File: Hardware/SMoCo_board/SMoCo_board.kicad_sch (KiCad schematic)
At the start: 37 parts, among them J1 Conn_01x02, J2 Conn_01x02, J3 Conn_01x02, J4 Conn_01x02, J5 Conn_01x06, J6 Conn_01x02, J7 Conn_01x04, J8 Conn_01x02, Q1 Q_PMOS, U1 STM32F072C8T6, U2 VNH7040AYTR, U3 SN65HVD232, U4 AP63203WU

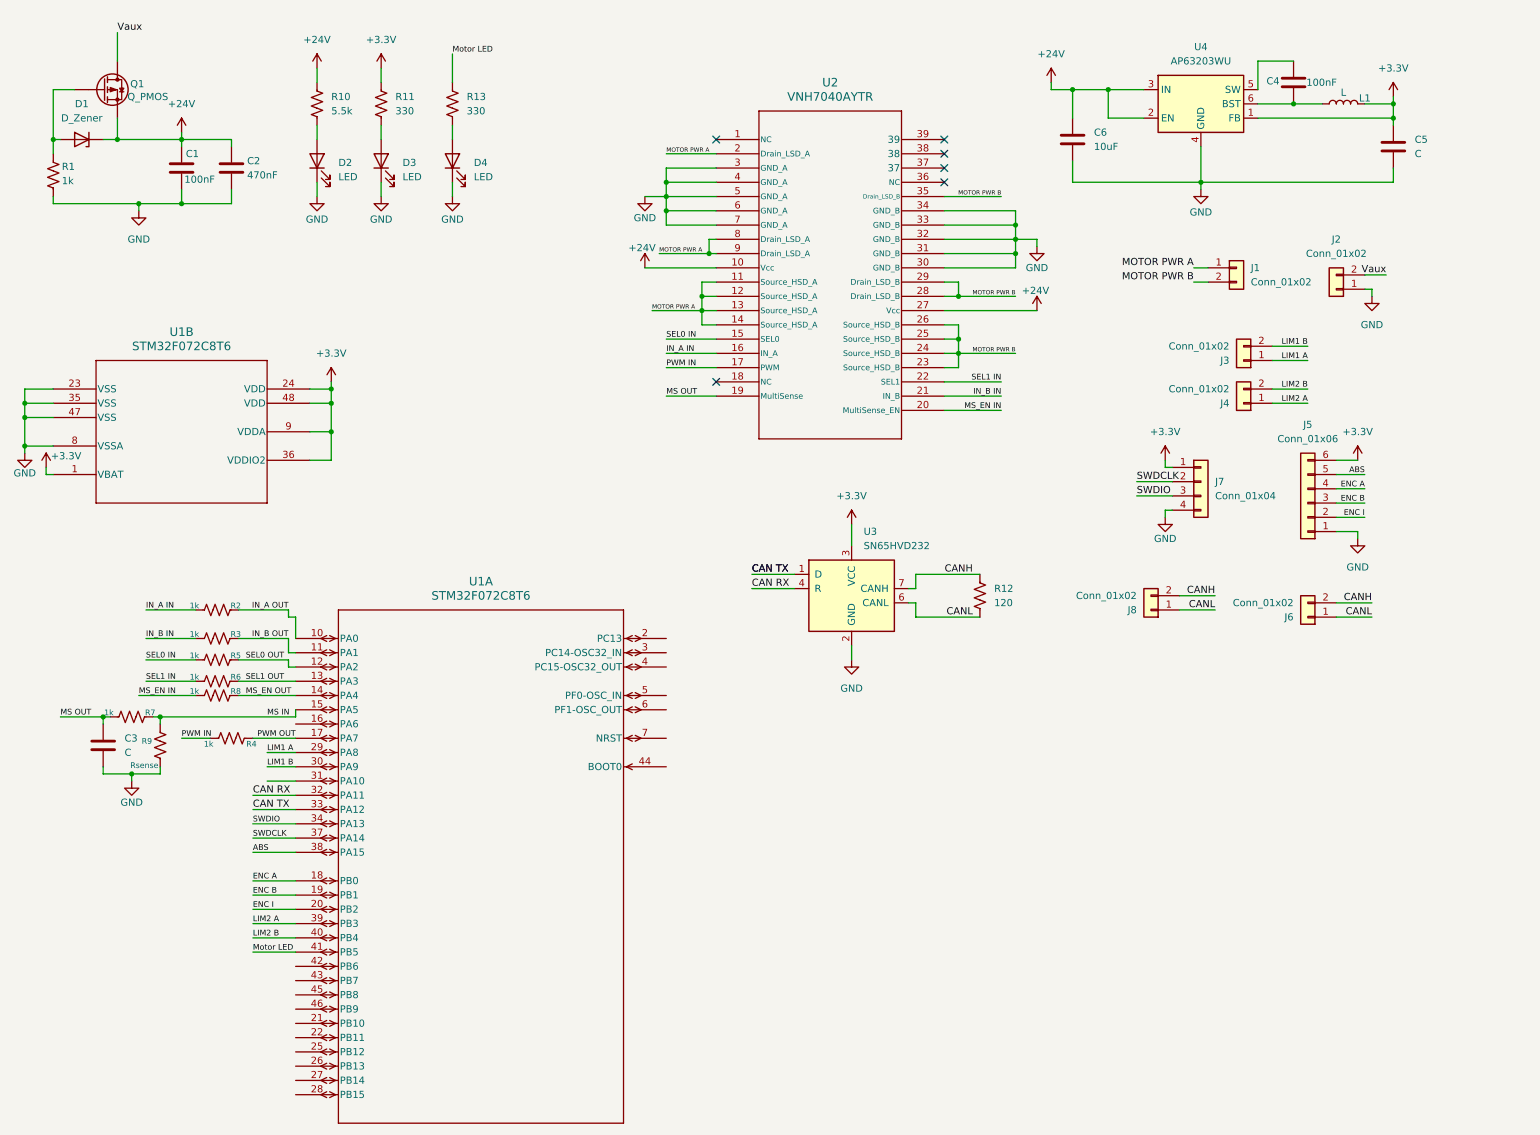
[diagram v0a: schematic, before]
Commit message: fix bug
this was gavin lmao
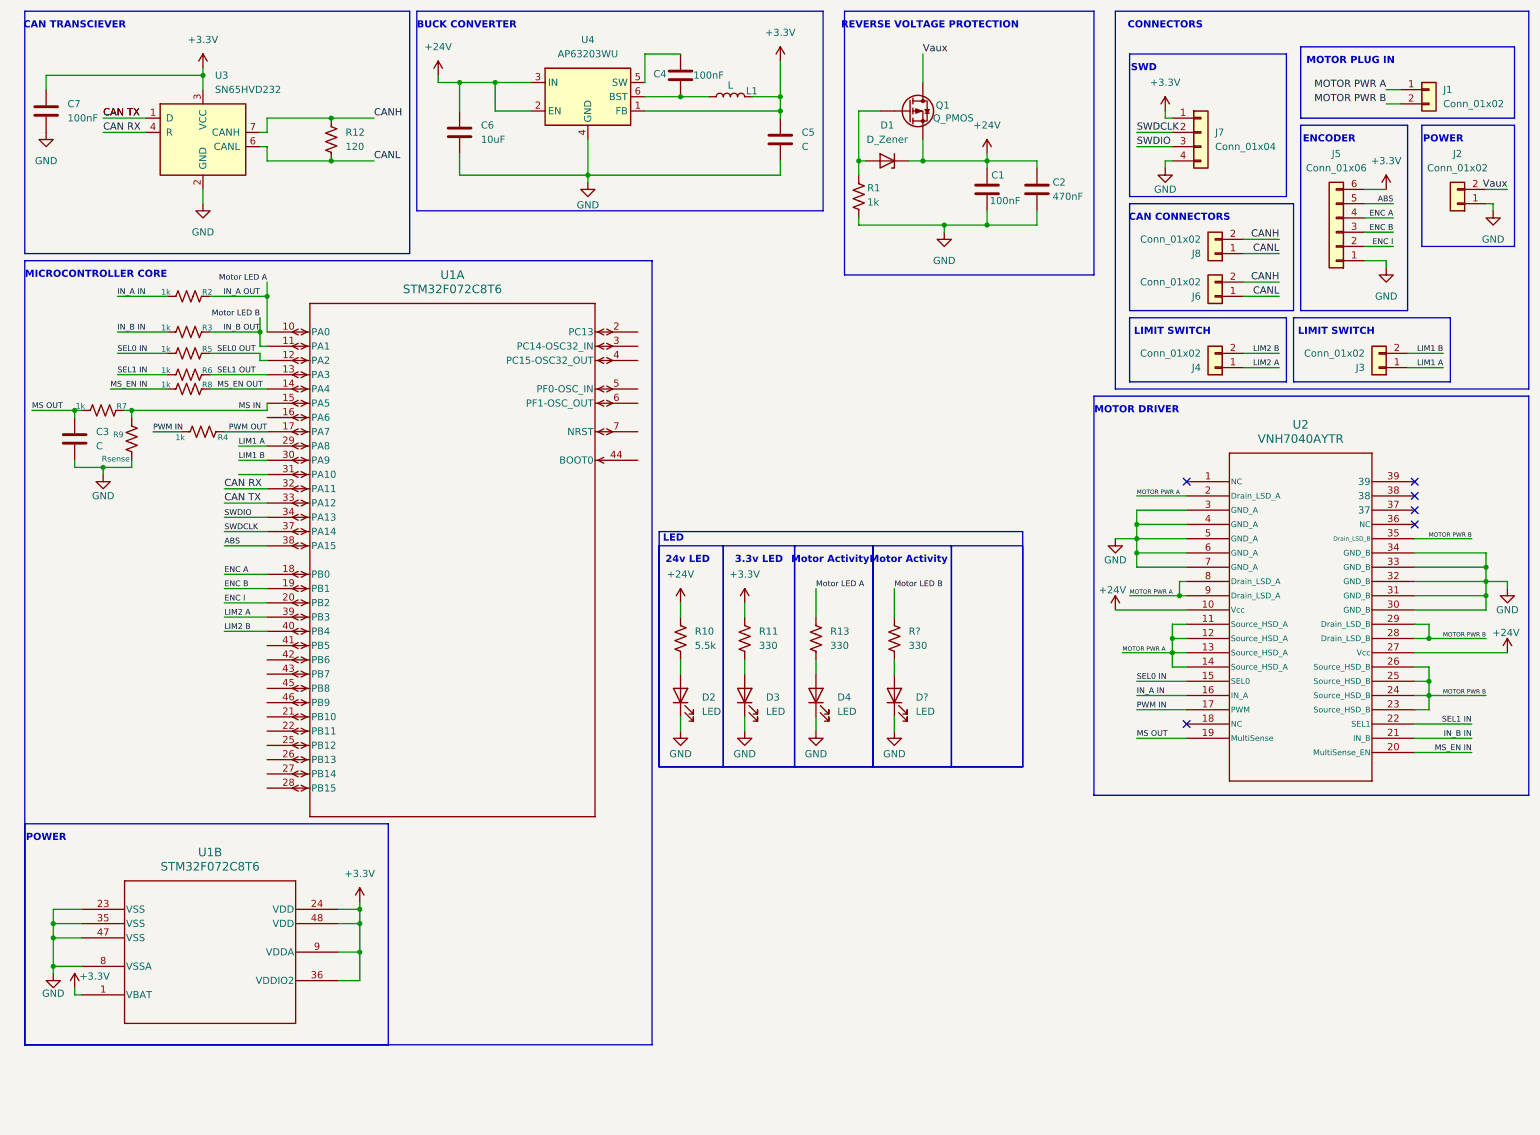
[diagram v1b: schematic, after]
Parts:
- added C7: 100nF, symbol Device:C
- added D?: LED, symbol Device:LED
- added R?: 330, symbol Device:R_US
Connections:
- net +3.3V: now also C7.1
- net GND: now also C7.2, D?.1 (K)
- net IN_A OUT: now also R13.1
- net IN_B OUT: now also R?.1
- net Motor LED: no longer names the net of U1.41 (PB5)
- net Motor LED: no longer R13.1
- new net: D?.2 (A), R?.2
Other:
- note added: "24v LED"
- note added: "3.3v LED"
- note added: "BUCK CONVERTER"
- note added: "CAN CONNECTORS"
- note added: "CAN TRANSCIEVER"
- note added: "CONNECTORS"
- note added: "ENCODER"
- note added: "LED"
- note added: "LIMIT SWITCH"
- note added: "MICROCONTROLLER CORE"
- note added: "MOTOR DRIVER"
- note added: "MOTOR PLUG IN"
- note added: "Motor Activity"
- note added: "POWER"
- note added: "REVERSE VOLTAGE PROTECTION"
- note added: "SWD"
- moved on the sheet: C1, C2, C3, C4, C5, C6, D1, D2, D3, D4, J1, J2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
